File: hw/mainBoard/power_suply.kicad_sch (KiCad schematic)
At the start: 3 parts, among them U2 AMS1117-3.3

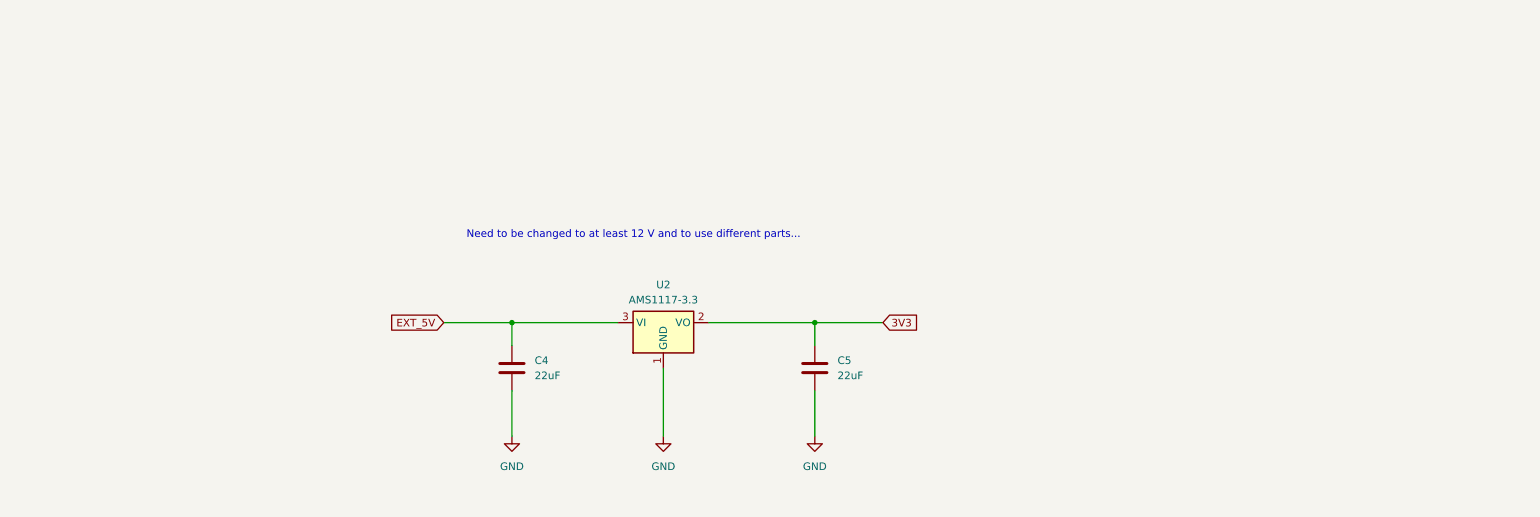
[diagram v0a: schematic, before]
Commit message: hw
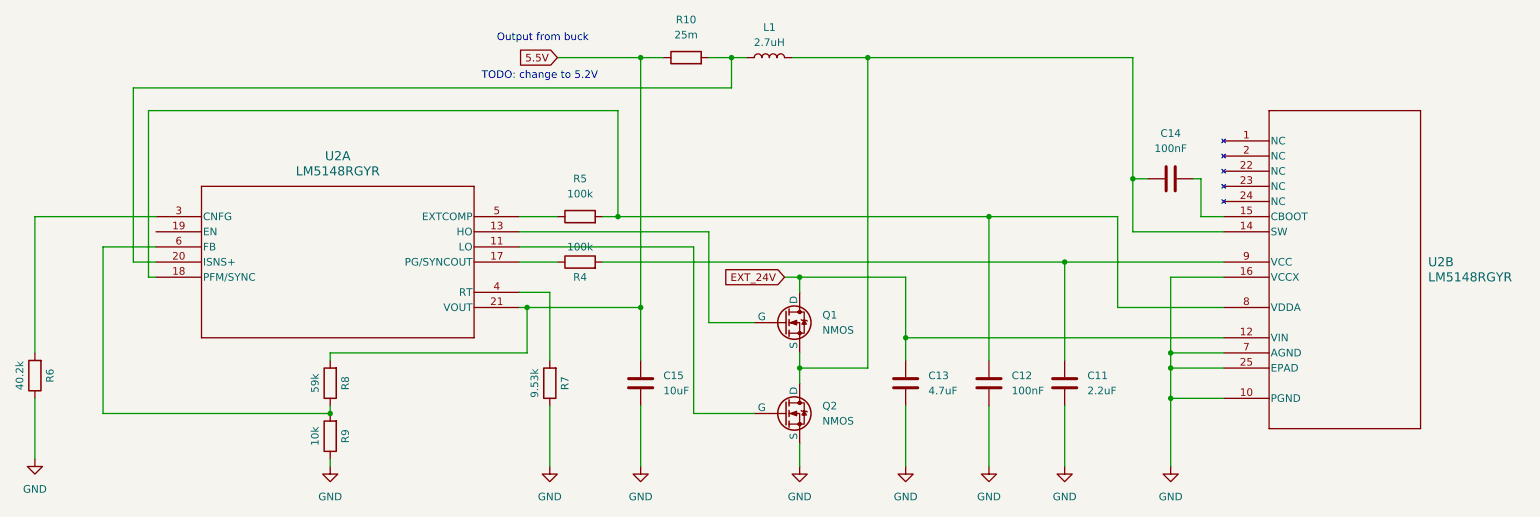
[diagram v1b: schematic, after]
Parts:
- removed C4, C5: 22uF, symbol Device:C
- removed U2: AMS1117-3.3, Package_TO_SOT_SMD:SOT-223-3_TabPin2, symbol Regulator_Linear:AMS1117-3.3
- added C11: 2.2uF, symbol Device:C
- added C12, C14: 100nF, symbol Device:C
- added C13: 4.7uF, symbol Device:C
- added C15: 10uF, symbol Device:C
- added L1: 2.7uH, symbol Device:L
- added Q1, Q2: NMOS, symbol Simulation_SPICE:NMOS
- added R10: 25m, symbol Device:R
- added R4, R5: 100k, symbol Device:R
- added R6: 40.2k, symbol Device:R
- added R7: 9.53k, symbol Device:R
- added R8: 59k, symbol Device:R
- added R9: 10k, symbol Device:R
- added U2: LM5148RGYR, VQFN24_RGY_TEX, symbol LM5148:LM5148RGYR
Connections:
- net GND: now also C11.2, C12.2, C13.2, C15.2, Q2.3 (S), R6.1, R7.1, R9.1, U2.10 (PGND), U2.16 (VCCX), U2.25 (EPAD), U2.7 (AGND)
- new net: R6.2, U2.3 (CNFG)
- new net: C14.1, L1.2, Q1.3 (S), Q2.1 (D), U2.14 (SW)
- new net: C14.2, U2.15 (CBOOT)
- new net: C12.1, R5.2, U2.18 (PFM/SYNC), U2.8 (VDDA)
- new net: C11.1, R4.2, U2.9 (VCC)
- new net: R8.1, R9.2, U2.6 (FB)
- new net: L1.1, R10.2, U2.20 (ISNS+)
- new net: Q1.2 (G), U2.13 (HO)
- new net: Q2.2 (G), U2.11 (LO)
- new net: R4.1, U2.17 (PG/SYNCOUT)
- new net: R7.2, U2.4 (RT)
- new net: R5.1, U2.5 (EXTCOMP)
- new net 5.5V: C15.1, R10.1, R8.2, U2.21 (VOUT)
- new net EXT_24V: C13.1, Q1.1 (D), U2.12 (VIN)
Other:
- note added: "Output from buck"
- note added: "TODO: change to 5.2V"
- note removed: "Need to be changed to at least 12 V and to use different parts..."
